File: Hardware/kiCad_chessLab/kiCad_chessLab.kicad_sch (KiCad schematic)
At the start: 0 parts

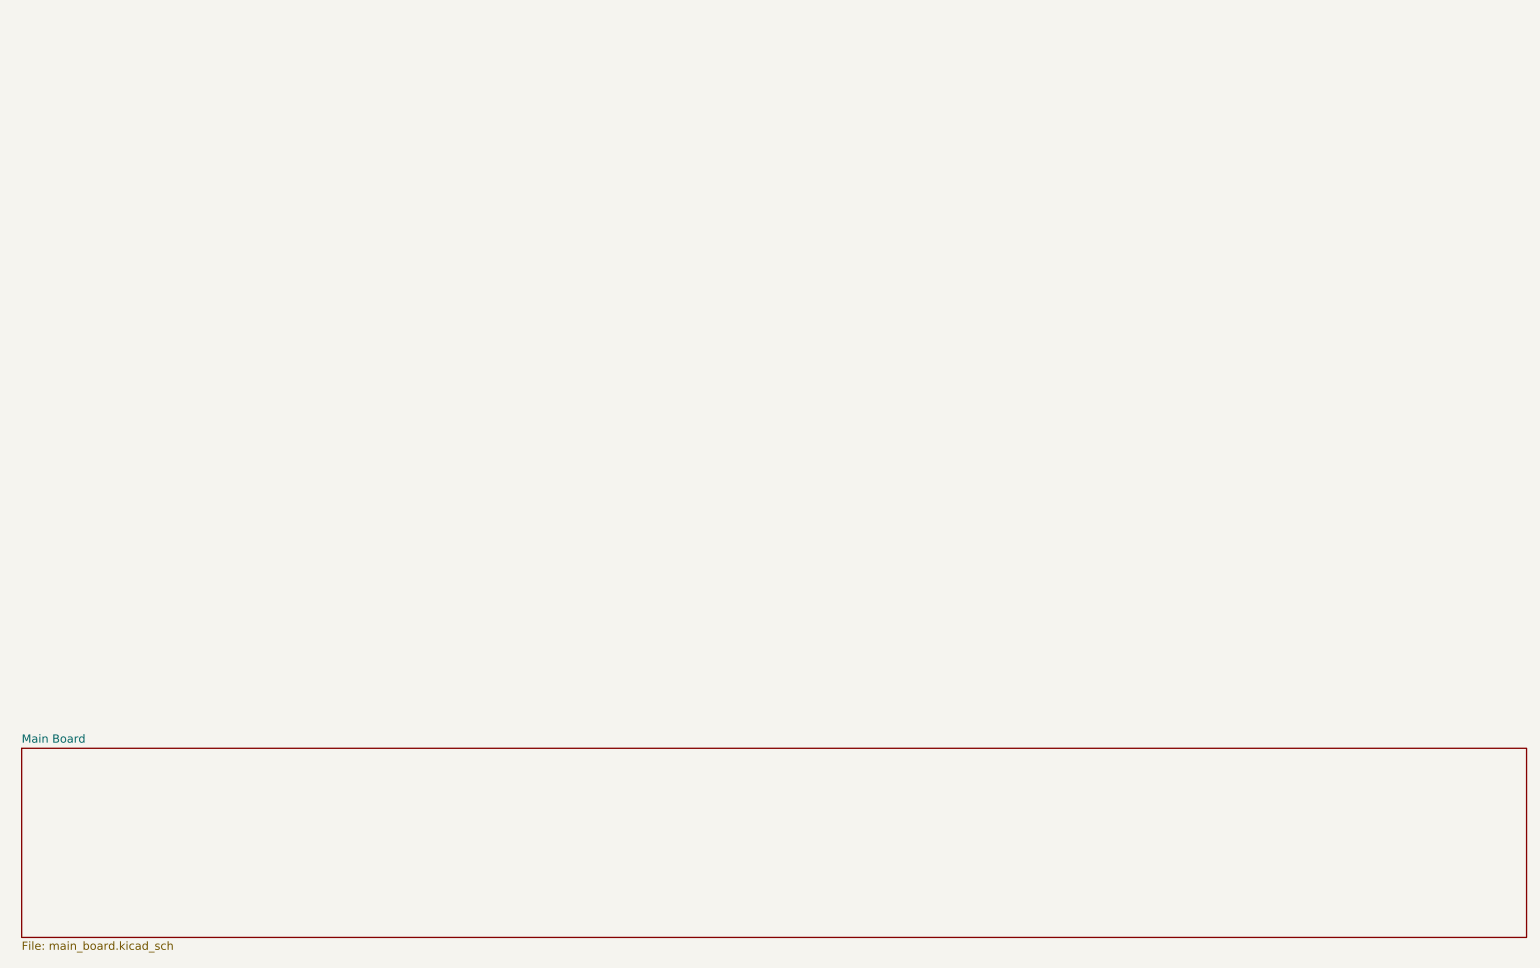
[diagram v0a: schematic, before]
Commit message: Usb c new design
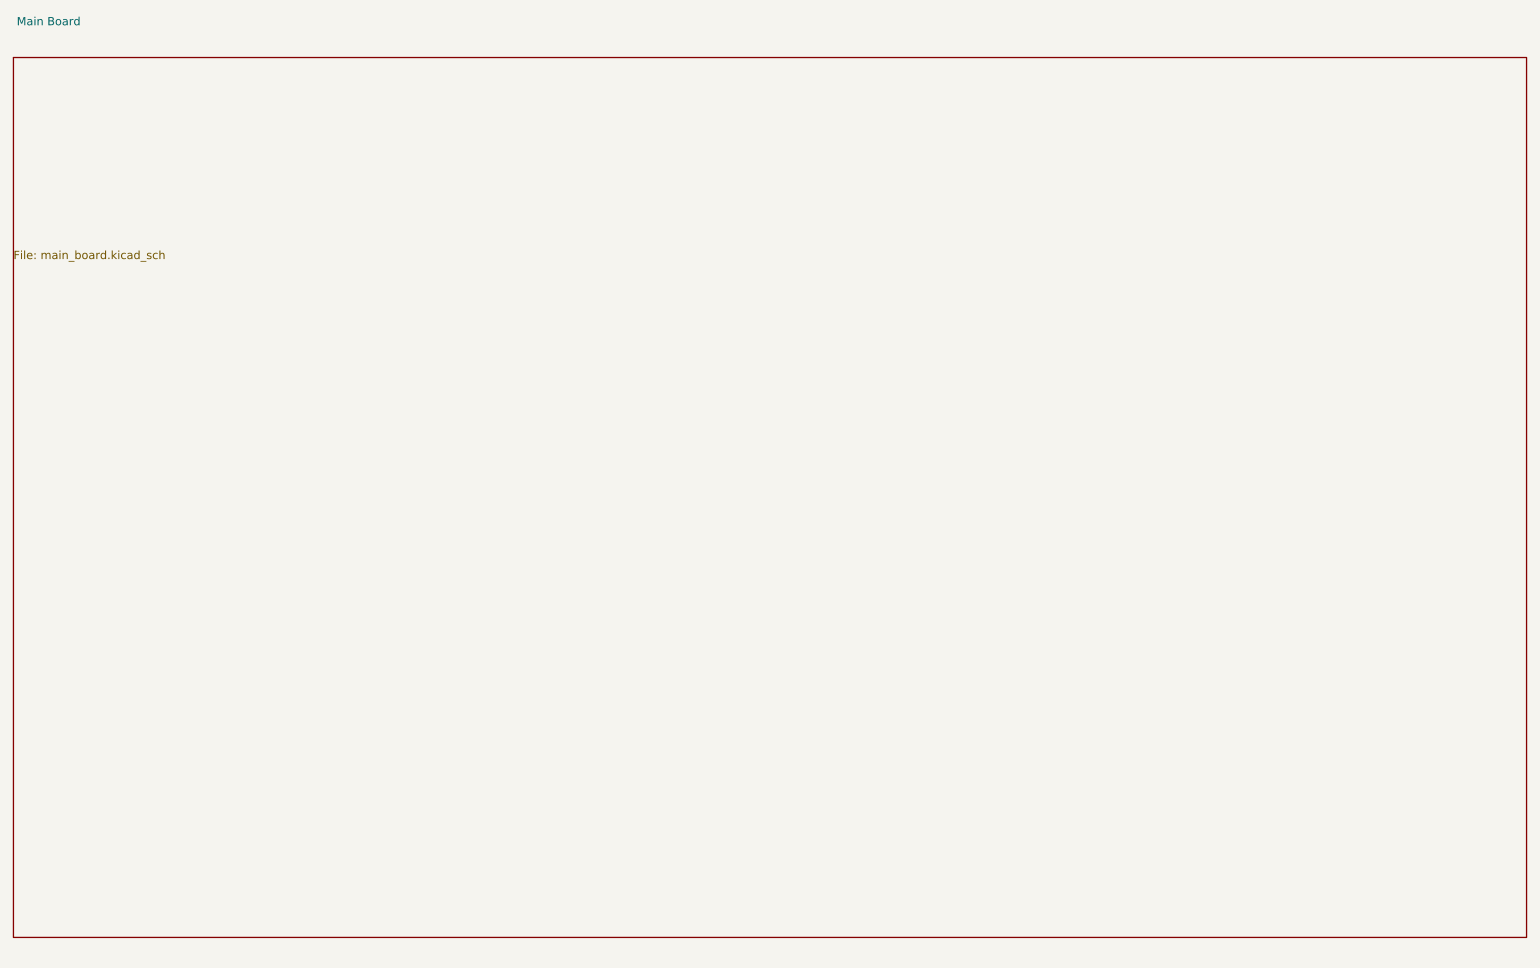
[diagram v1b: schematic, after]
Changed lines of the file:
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@@
 	)
 	(sheet
-		(at 22.86 129.54)
-		(size 232.41 29.21)
+		(at 21.59 22.86)
+		(size 233.68 135.89)
 		(exclude_from_sim no)
 		(in_bom yes)
 		(on_board yes)
 		(dnp no)
-		(fields_autoplaced yes)
 		(stroke
 			(width 0.1524)
@@
 		)
 		(property "Sheetname" "Main Board"
-			(at 22.86 128.8284 0)
+			(at 22.098 18.034 0)
 			(show_name no)
 			(do_not_autoplace no)
@@
 		)
 		(property "Sheetfile" "main_board.kicad_sch"
-			(at 22.86 159.3346 0)
+			(at 21.59 52.6546 0)
 			(show_name no)
 			(do_not_autoplace no)
